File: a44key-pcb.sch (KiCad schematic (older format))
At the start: 60 parts

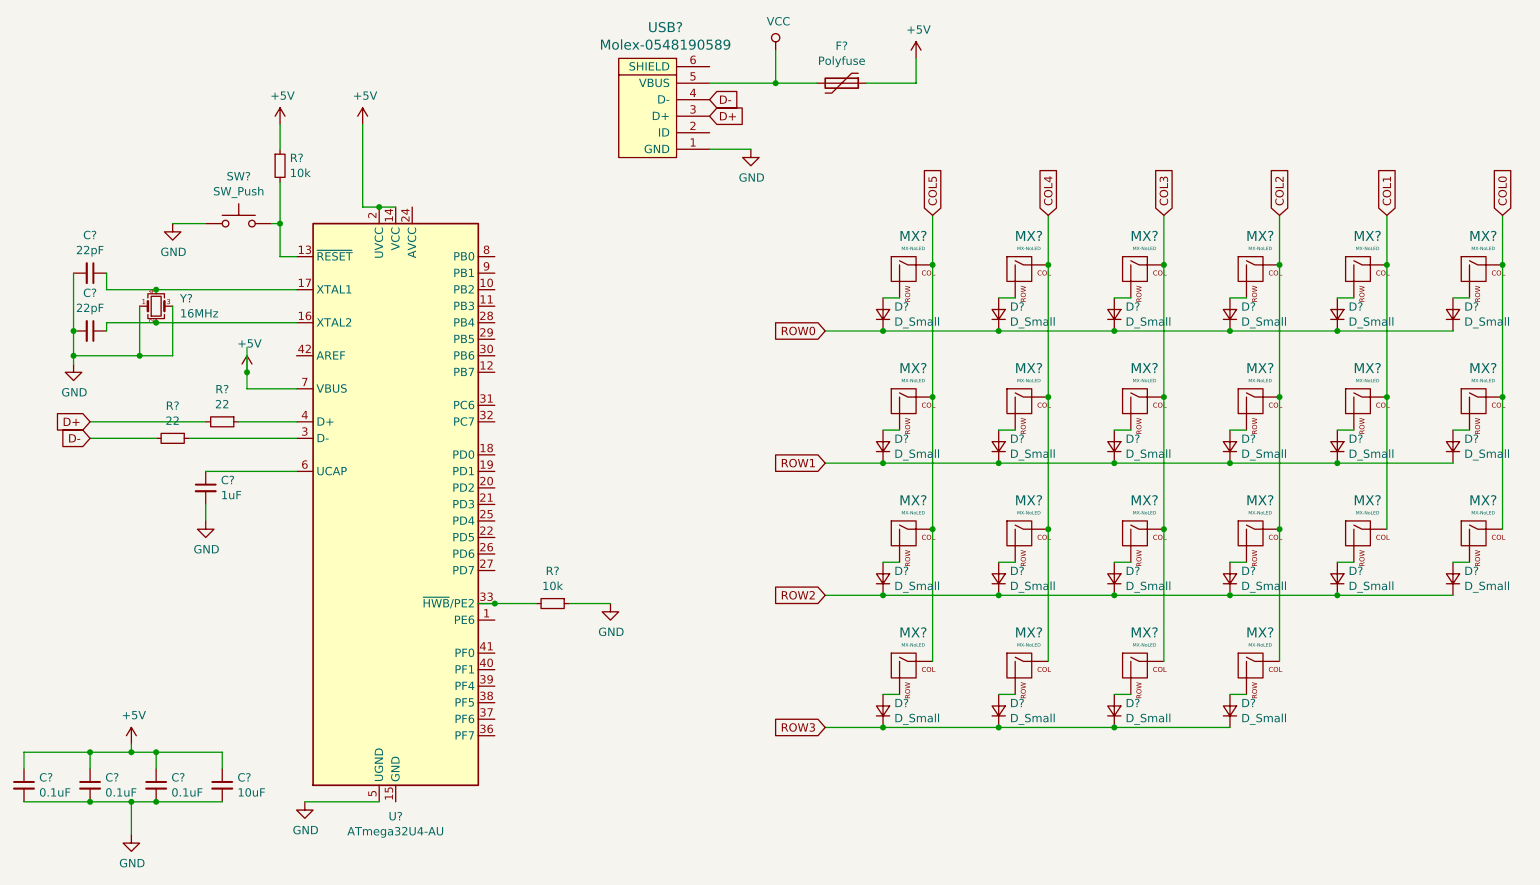
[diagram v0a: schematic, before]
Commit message: Submodules added
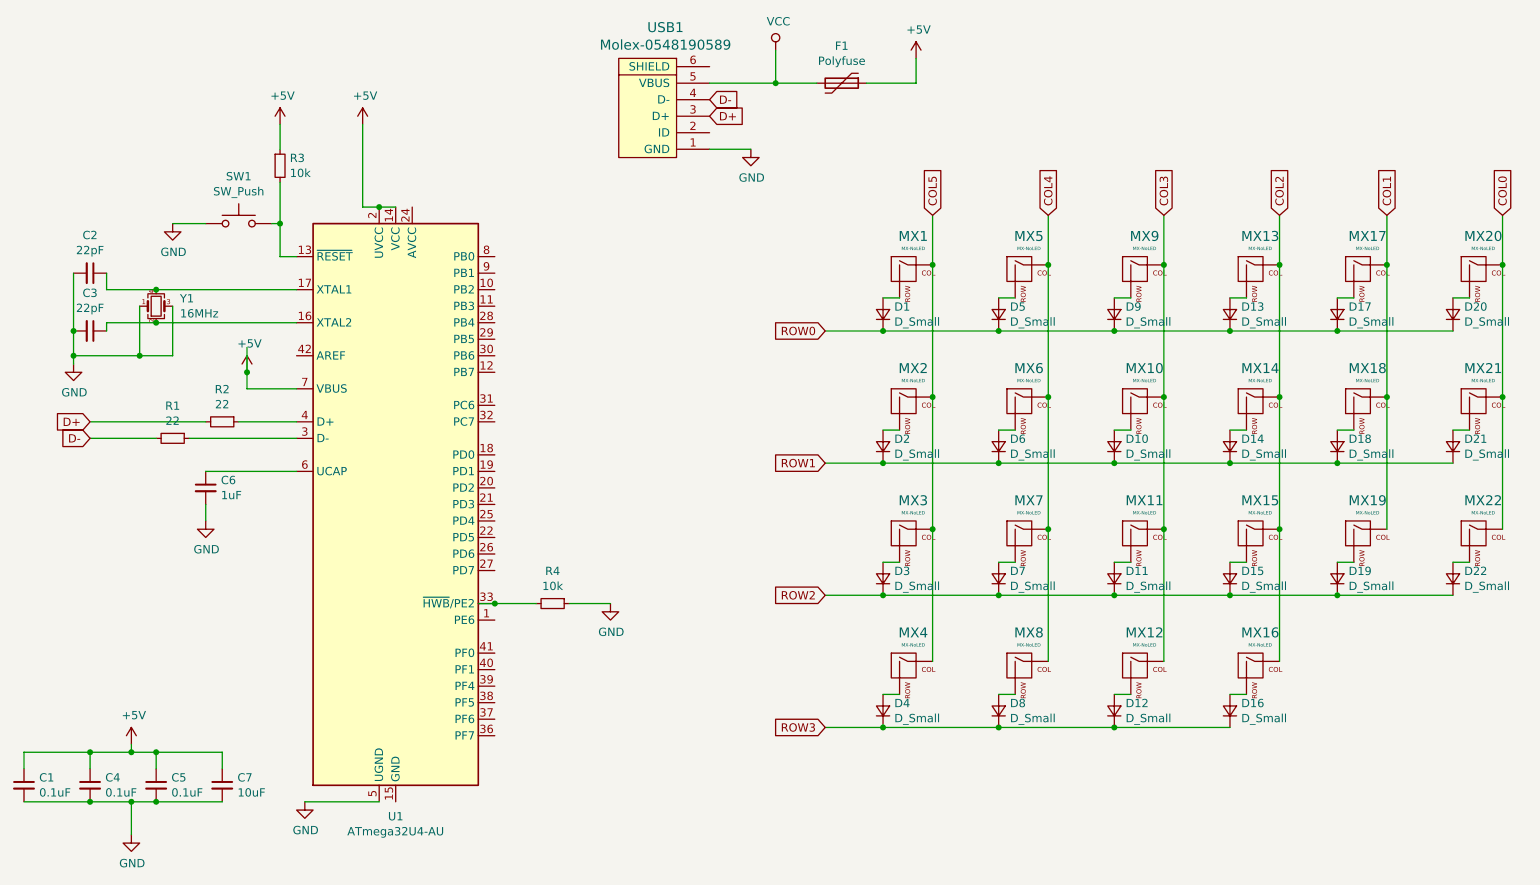
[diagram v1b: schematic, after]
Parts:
- C1, C2, C3, C4, C5, C6, C7: renamed from C?; footprint (none) -> Capacitor_SMD:C_0805_2012Metric
- D1, D10, D11, D12, D13, D14, D15, D16, D17, D18, D19, D2, D20, D21, D22, D3, D4, D5, D6, D7, D8, D9: renamed from D?; footprint (none) -> MX_Alps_Hybrid:MX-1U-NoLED
- F1: renamed from F?; footprint (none) -> MX_Alps_Hybrid:MX-1U-NoLED
- MX1, MX10, MX11, MX12, MX13, MX14, MX15, MX16, MX17, MX18, MX19, MX2, MX20, MX21, MX22, MX3, MX4, MX5, MX6, MX7, MX8, MX9: renamed from MX?; footprint (none) -> MX_Alps_Hybrid:MX-1U-NoLED
- R1, R2, R3, R4: renamed from R?; footprint (none) -> Resistor_SMD:R_0805_2012Metric
- SW1: renamed from SW?; footprint (none) -> random-keyboard-parts:SKQG-1155865
- USB1: renamed from USB?; footprint (none) -> random-keyboard-parts:Molex-0548190589
- Y1: renamed from Y?; footprint (none) -> Crystal:Crystal_SMD_3225-4Pin_3.2x2.5mm_HandSoldering
- gave numbers to parts that had none: 1

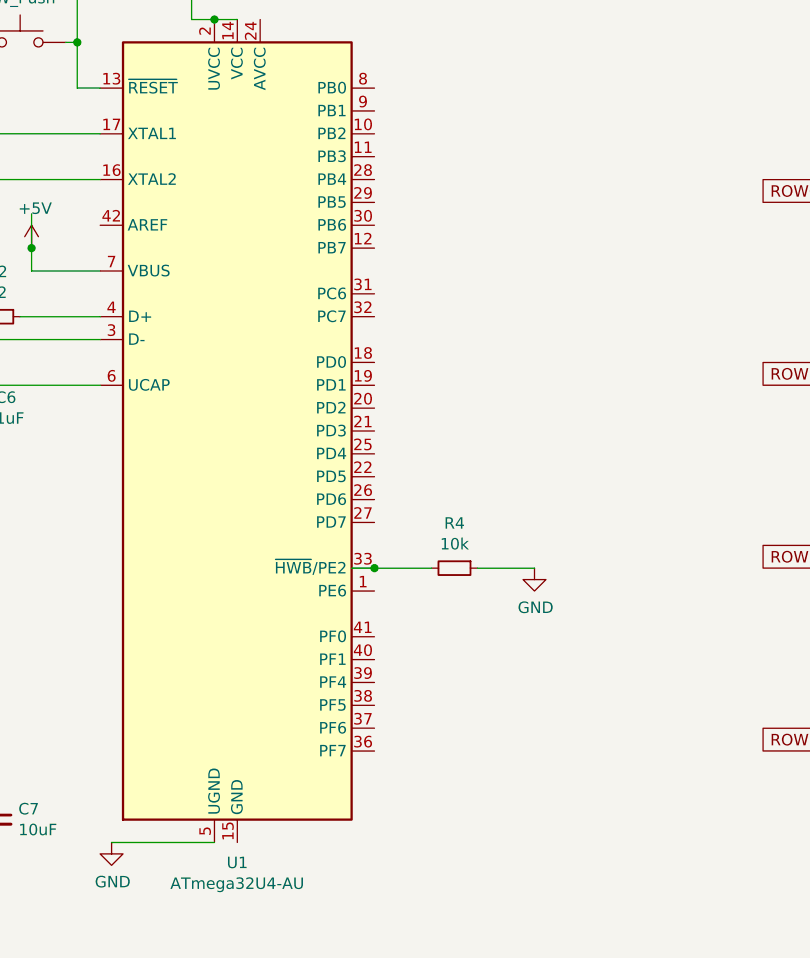
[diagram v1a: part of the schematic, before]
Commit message: Submodules added
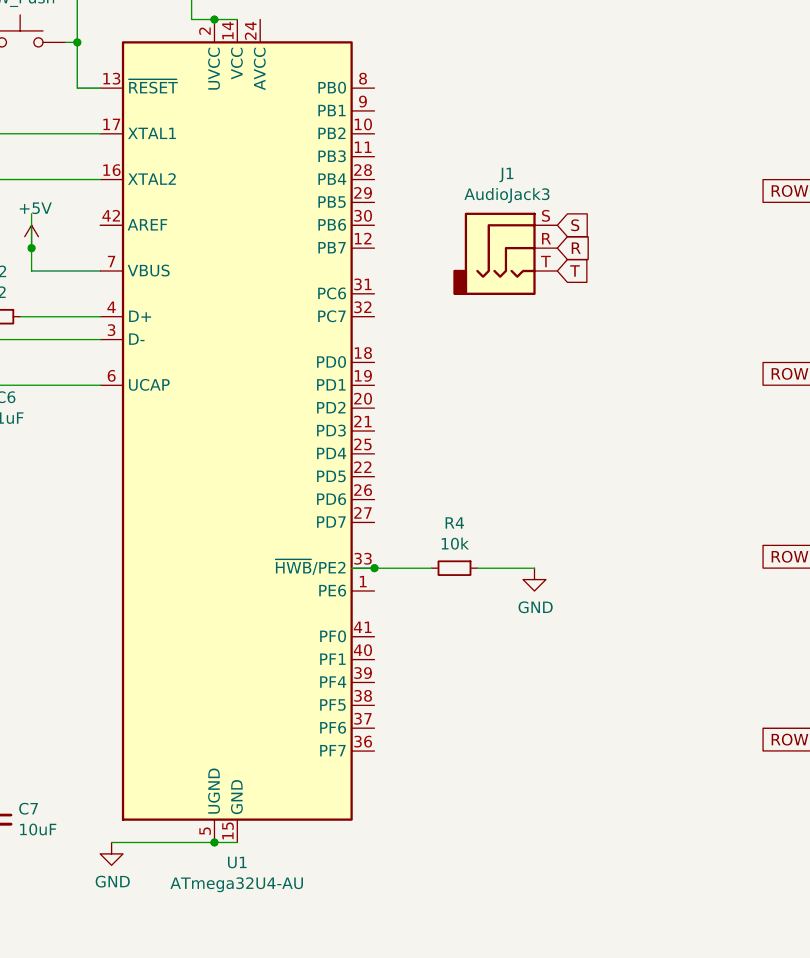
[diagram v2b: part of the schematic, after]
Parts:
- added J1: AudioJack3, Connector_Audio:Jack_3.5mm_CUI_SJ1-3535NG_Horizontal, symbol Connector:AudioJack3
- D1, D10, D11, D12, D13, D14, D15, D16, D17, D18, D19, D2, D20, D21, D22, D3, D4, D5, D6, D7, D8, D9: footprint MX_Alps_Hybrid:MX-1U-NoLED -> Diode_SMD:D_SOD-123
- F1: footprint MX_Alps_Hybrid:MX-1U-NoLED -> Fuse:Fuse_1206_3216Metric
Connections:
- net GND: now also U1.15 (GND), U1.23 (GND), U1.35 (GND), U1.43 (GND)
- new net R: J1.R
- new net S: J1.S
- new net T: J1.T
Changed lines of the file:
@@
 F 0 "F1" V 6075 1200 50  0000 C CNN
 F 1 "Polyfuse" V 6166 1200 50  0000 C CNN
-F 2 "MX_Alps_Hybrid:MX-1U-NoLED" H 6350 1000 50  0001 L CNN
+F 2 "Fuse:Fuse_1206_3216Metric" H 6350 1000 50  0001 L CNN
 F 3 "~" H 6300 1200 50  0001 C CNN
 	1    6300 1200
@@
 F 0 "D1" V 6596 2532 50  0000 R CNN
 F 1 "D_Small" V 6505 2532 50  0000 R CNN
-F 2 "MX_Alps_Hybrid:MX-1U-NoLED" V 6550 2600 50  0001 C CNN
+F 2 "Diode_SMD:D_SOD-123" V 6550 2600 50  0001 C CNN
 F 3 "~" V 6550 2600 50  0001 C CNN
 	1    6550 2600
@@
 F 0 "D5" V 7296 2532 50  0000 R CNN
 F 1 "D_Small" V 7205 2532 50  0000 R CNN
-F 2 "MX_Alps_Hybrid:MX-1U-NoLED" V 7250 2600 50  0001 C CNN
+F 2 "Diode_SMD:D_SOD-123" V 7250 2600 50  0001 C CNN
 F 3 "~" V 7250 2600 50  0001 C CNN
 	1    7250 2600
@@
 F 0 "D2" V 6596 3332 50  0000 R CNN
 F 1 "D_Small" V 6505 3332 50  0000 R CNN
-F 2 "MX_Alps_Hybrid:MX-1U-NoLED" V 6550 3400 50  0001 C CNN
+F 2 "Diode_SMD:D_SOD-123" V 6550 3400 50  0001 C CNN
 F 3 "~" V 6550 3400 50  0001 C CNN
 	1    6550 3400
@@
 F 0 "D6" V 7296 3332 50  0000 R CNN
 F 1 "D_Small" V 7205 3332 50  0000 R CNN
-F 2 "MX_Alps_Hybrid:MX-1U-NoLED" V 7250 3400 50  0001 C CNN
+F 2 "Diode_SMD:D_SOD-123" V 7250 3400 50  0001 C CNN
 F 3 "~" V 7250 3400 50  0001 C CNN
 	1    7250 3400
@@
 F 0 "D9" V 7996 2532 50  0000 R CNN
 F 1 "D_Small" V 7905 2532 50  0000 R CNN
-F 2 "MX_Alps_Hybrid:MX-1U-NoLED" V 7950 2600 50  0001 C CNN
+F 2 "Diode_SMD:D_SOD-123" V 7950 2600 50  0001 C CNN
 F 3 "~" V 7950 2600 50  0001 C CNN
 	1    7950 2600
@@
 F 0 "D13" V 8696 2532 50  0000 R CNN
 F 1 "D_Small" V 8605 2532 50  0000 R CNN
-F 2 "MX_Alps_Hybrid:MX-1U-NoLED" V 8650 2600 50  0001 C CNN
+F 2 "Diode_SMD:D_SOD-123" V 8650 2600 50  0001 C CNN
 F 3 "~" V 8650 2600 50  0001 C CNN
 	1    8650 2600
@@
 F 0 "D10" V 7996 3332 50  0000 R CNN
 F 1 "D_Small" V 7905 3332 50  0000 R CNN
-F 2 "MX_Alps_Hybrid:MX-1U-NoLED" V 7950 3400 50  0001 C CNN
+F 2 "Diode_SMD:D_SOD-123" V 7950 3400 50  0001 C CNN
 F 3 "~" V 7950 3400 50  0001 C CNN
 	1    7950 3400
@@
 F 0 "D14" V 8696 3332 50  0000 R CNN
 F 1 "D_Small" V 8605 3332 50  0000 R CNN
-F 2 "MX_Alps_Hybrid:MX-1U-NoLED" V 8650 3400 50  0001 C CNN
+F 2 "Diode_SMD:D_SOD-123" V 8650 3400 50  0001 C CNN
 F 3 "~" V 8650 3400 50  0001 C CNN
 	1    8650 3400
@@
 F 0 "D3" V 6596 4132 50  0000 R CNN
 F 1 "D_Small" V 6505 4132 50  0000 R CNN
-F 2 "MX_Alps_Hybrid:MX-1U-NoLED" V 6550 4200 50  0001 C CNN
+F 2 "Diode_SMD:D_SOD-123" V 6550 4200 50  0001 C CNN
 F 3 "~" V 6550 4200 50  0001 C CNN
 	1    6550 4200
@@
 F 0 "D7" V 7296 4132 50  0000 R CNN
 F 1 "D_Small" V 7205 4132 50  0000 R CNN
-F 2 "MX_Alps_Hybrid:MX-1U-NoLED" V 7250 4200 50  0001 C CNN
+F 2 "Diode_SMD:D_SOD-123" V 7250 4200 50  0001 C CNN
 F 3 "~" V 7250 4200 50  0001 C CNN
 	1    7250 4200
@@
 F 0 "D4" V 6596 4932 50  0000 R CNN
 F 1 "D_Small" V 6505 4932 50  0000 R CNN
-F 2 "MX_Alps_Hybrid:MX-1U-NoLED" V 6550 5000 50  0001 C CNN
+F 2 "Diode_SMD:D_SOD-123" V 6550 5000 50  0001 C CNN
 F 3 "~" V 6550 5000 50  0001 C CNN
 	1    6550 5000
@@
 F 0 "D8" V 7296 4932 50  0000 R CNN
 F 1 "D_Small" V 7205 4932 50  0000 R CNN
-F 2 "MX_Alps_Hybrid:MX-1U-NoLED" V 7250 5000 50  0001 C CNN
+F 2 "Diode_SMD:D_SOD-123" V 7250 5000 50  0001 C CNN
 F 3 "~" V 7250 5000 50  0001 C CNN
 	1    7250 5000
@@
 F 0 "D11" V 7996 4132 50  0000 R CNN
 F 1 "D_Small" V 7905 4132 50  0000 R CNN
-F 2 "MX_Alps_Hybrid:MX-1U-NoLED" V 7950 4200 50  0001 C CNN
+F 2 "Diode_SMD:D_SOD-123" V 7950 4200 50  0001 C CNN
 F 3 "~" V 7950 4200 50  0001 C CNN
 	1    7950 4200
@@
 F 0 "D15" V 8696 4132 50  0000 R CNN
 F 1 "D_Small" V 8605 4132 50  0000 R CNN
-F 2 "MX_Alps_Hybrid:MX-1U-NoLED" V 8650 4200 50  0001 C CNN
+F 2 "Diode_SMD:D_SOD-123" V 8650 4200 50  0001 C CNN
 F 3 "~" V 8650 4200 50  0001 C CNN
 	1    8650 4200
@@
 F 0 "D12" V 7996 4932 50  0000 R CNN
 F 1 "D_Small" V 7905 4932 50  0000 R CNN
-F 2 "MX_Alps_Hybrid:MX-1U-NoLED" V 7950 5000 50  0001 C CNN
+F 2 "Diode_SMD:D_SOD-123" V 7950 5000 50  0001 C CNN
 F 3 "~" V 7950 5000 50  0001 C CNN
 	1    7950 5000
@@
 F 0 "D16" V 8696 4932 50  0000 R CNN
 F 1 "D_Small" V 8605 4932 50  0000 R CNN
-F 2 "MX_Alps_Hybrid:MX-1U-NoLED" V 8650 5000 50  0001 C CNN
+F 2 "Diode_SMD:D_SOD-123" V 8650 5000 50  0001 C CNN
 F 3 "~" V 8650 5000 50  0001 C CNN
 	1    8650 5000
@@
 F 0 "D17" V 9346 2532 50  0000 R CNN
 F 1 "D_Small" V 9255 2532 50  0000 R CNN
-F 2 "MX_Alps_Hybrid:MX-1U-NoLED" V 9300 2600 50  0001 C CNN
+F 2 "Diode_SMD:D_SOD-123" V 9300 2600 50  0001 C CNN
 F 3 "~" V 9300 2600 50  0001 C CNN
 	1    9300 2600
@@
 F 0 "D20" V 10046 2532 50  0000 R CNN
 F 1 "D_Small" V 9955 2532 50  0000 R CNN
-F 2 "MX_Alps_Hybrid:MX-1U-NoLED" V 10000 2600 50  0001 C CNN
+F 2 "Diode_SMD:D_SOD-123" V 10000 2600 50  0001 C CNN
 F 3 "~" V 10000 2600 50  0001 C CNN
 	1    10000 2600
@@
 F 0 "D18" V 9346 3332 50  0000 R CNN
 F 1 "D_Small" V 9255 3332 50  0000 R CNN
-F 2 "MX_Alps_Hybrid:MX-1U-NoLED" V 9300 3400 50  0001 C CNN
+F 2 "Diode_SMD:D_SOD-123" V 9300 3400 50  0001 C CNN
 F 3 "~" V 9300 3400 50  0001 C CNN
 	1    9300 3400
@@
 F 0 "D21" V 10046 3332 50  0000 R CNN
 F 1 "D_Small" V 9955 3332 50  0000 R CNN
-F 2 "MX_Alps_Hybrid:MX-1U-NoLED" V 10000 3400 50  0001 C CNN
+F 2 "Diode_SMD:D_SOD-123" V 10000 3400 50  0001 C CNN
 F 3 "~" V 10000 3400 50  0001 C CNN
 	1    10000 3400
@@
 F 0 "D19" V 9346 4132 50  0000 R CNN
 F 1 "D_Small" V 9255 4132 50  0000 R CNN
-F 2 "MX_Alps_Hybrid:MX-1U-NoLED" V 9300 4200 50  0001 C CNN
+F 2 "Diode_SMD:D_SOD-123" V 9300 4200 50  0001 C CNN
 F 3 "~" V 9300 4200 50  0001 C CNN
 	1    9300 4200
@@
 F 0 "D22" V 10046 4132 50  0000 R CNN
 F 1 "D_Small" V 9955 4132 50  0000 R CNN
-F 2 "MX_Alps_Hybrid:MX-1U-NoLED" V 10000 4200 50  0001 C CNN
+F 2 "Diode_SMD:D_SOD-123" V 10000 4200 50  0001 C CNN
 F 3 "~" V 10000 4200 50  0001 C CNN
 	1    10000 4200
@@
 Text GLabel 6200 5100 0    50   Input ~ 0
 ROW3
+$Comp
+L Connector:AudioJack3 J1
+U 1 1 6186D5DF
+P 4800 2950
+F 0 "J1" H 4782 3275 50  0000 C CNN
+F 1 "AudioJack3" H 4782 3184 50  0000 C CNN
+F 2 "Connector_Audio:Jack_3.5mm_CUI_SJ1-3535NG_Horizontal" H 4800 2950 50  0001 C CNN
+F 3 "~" H 4800 2950 50  0001 C CNN
+	1    4800 2950
+	1    0    0    -1
+$EndComp
+Text GLabel 5000 2850 2    50   Input ~ 0
+S
+Text GLabel 5000 2950 2    50   Input ~ 0
+R
+Text GLabel 5000 3050 2    50   Input ~ 0
+T
+Wire Wire Line
+	3500 5550 3600 5550
+Connection ~ 3500 5550
 $EndSCHEMATC
